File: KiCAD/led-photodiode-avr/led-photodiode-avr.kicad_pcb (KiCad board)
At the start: 4 copper layers, 68.6 x 80 mm, 68 parts, among them J1 Screw_Terminal_01x02, J2 Conn_02x08_Odd_Even, J3 ISP, J4 Conn_01x06_Pin, Q1 TTC1949, Q2 TTC1949, Q3 TTC1949, Q4 TTC1949, U1 REF3040AIDBZT, U10 AZ1117CH2-5.0, U2 AZ1117CH2-5.0, U3 OPA365xxD, U5 DDC112, U6 LTC1380, U7 ATmega328-A, U8 OPA365AIDR, U9 LTC2631, Y1 CO_16MHZ

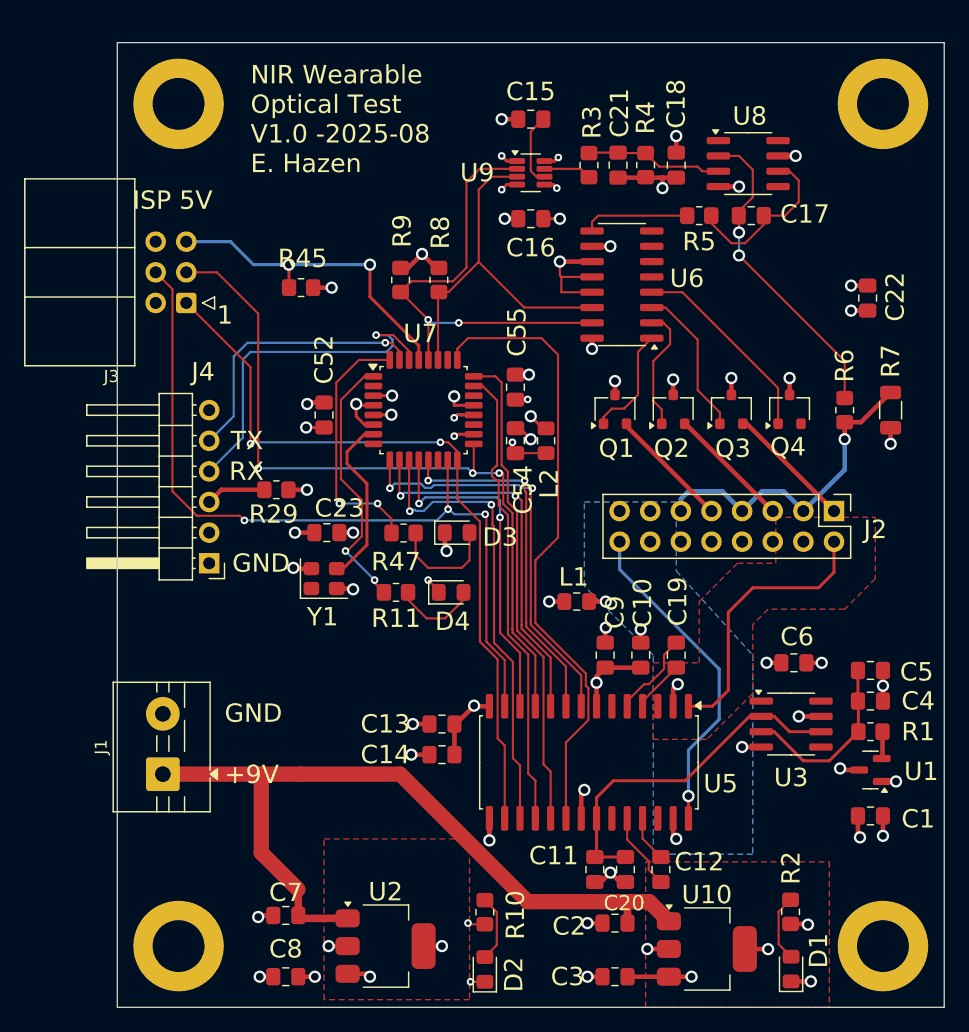
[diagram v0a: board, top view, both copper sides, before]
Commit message: more tests
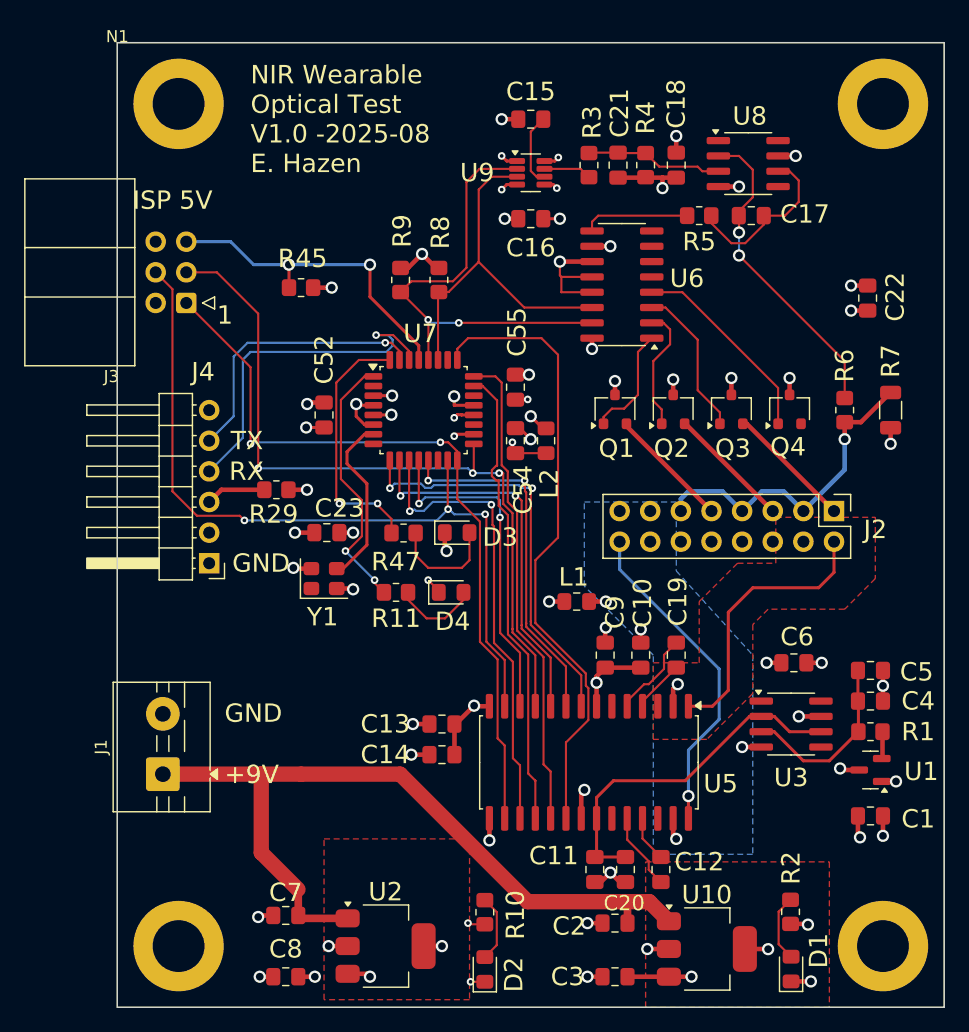
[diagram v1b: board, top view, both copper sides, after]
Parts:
- added N1: Optical_PCB, optical_pcb_model:optical_pcb, F.Cu at (116.8, 57.1)
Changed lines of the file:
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@@
 		)
 	)
+	(footprint "optical_pcb_model:optical_pcb"
+		(layer "F.Cu")
+		(at 116.84 57.15)
+		(property "Reference" "N1"
+			(at 0 -0.5 0)
+			(unlocked yes)
+			(layer "F.SilkS")
+			(effects
+				(font
+					(size 1 1)
+					(thickness 0.1)
+				)
+			)
+		)
+		(property "Value" "Optical_PCB"
+			(at 0 1 0)
+			(unlocked yes)
+			(layer "F.Fab")
+			(effects
+				(font
+					(size 1 1)
+					(thickness 0.15)
+				)
+			)
+		)
+		(property "Datasheet" "~"
+			(at 0 0 0)
+			(unlocked yes)
+			(layer "F.Fab")
+			(hide yes)
+			(effects
+				(font
+					(size 1 1)
+					(thickness 0.15)
+				)
+			)
+		)
+		(property "Description" "Housing"
+			(at 0 0 0)
+			(unlocked yes)
+			(layer "F.Fab")
+			(hide yes)
+			(effects
+				(font
+					(size 1 1)
+					(thickness 0.15)
+				)
+			)
+		)
+		(property ki_fp_filters "Enclosure* Housing*")
+		(sheetname "/")
+		(sheetfile "led-photodiode-avr.kicad_sch")
+		(attr smd)
+		(fp_rect
+			(start 0 0)
+			(end 68.58 80.01)
+			(stroke
+				(width 0.1)
+				(type default)
+			)
+			(fill no)
+			(layer "F.SilkS")
+		)
+		(fp_rect
+			(start 0 0)
+			(end 68.58 80.01)
+			(stroke
+				(width 0.1)
+				(type default)
+			)
+			(fill no)
+			(layer "User.2")
+		)
+		(fp_text user "${REFERENCE}"
+			(at 0 2.5 0)
+			(unlocked yes)
+			(layer "F.Fab")
+			(effects
+				(font
+					(size 1 1)
+					(thickness 0.15)
+				)
+			)
+		)
+		(pad "1" thru_hole circle
+			(at 5.08 5.08)
+			(size 4.572 4.572)
+			(drill 3.175)
+			(layers "*.Cu" "*.Mask")
+			(remove_unused_layers no)
+		)
+		(embedded_fonts no)
+		(model "${KIPRJMOD}/models/optical-carrier.wrl"
+			(offset
+				(xyz -169.545 55.88 12.065)
+			)
+			(scale
+				(xyz 0.392 0.392 0.392)
+			)
+			(rotate
+				(xyz -0 -0 -0)
+			)
+		)
+	)
 	(footprint "LED_SMD:LED_0805_2012Metric_Pad1.15x1.40mm_HandSolder"
 		(layer "F.Cu")
@@
 			(roundrect_rratio 0.25)
 			(net 6 "VCC")
-			(pinfunction "REF_SEL")
+			(pinfunction "CA1")
 			(pintype "passive")
 		)
@@
 		(layer "User.2")
 		(pts
+			(xy 116.84 57.15) (xy 121.92 62.23)
+		)
+		(height -6.604)
+		(orientation 0)
+		(format
+			(prefix "")
+			(suffix "")
+			(units 3)
+			(units_format 0)
+			(precision 4)
+			(suppress_zeroes yes)
+		)
+		(style
+			(thickness 0.1)
+			(arrow_length 1.27)
+			(text_position_mode 0)
+			(arrow_direction outward)
+			(extension_height 0.58642)
+			(extension_offset 0.5)
+			(keep_text_aligned yes)
+		)
+		(gr_text "0.2"
+			(at 119.38 49.396 0)
+			(layer "User.2")
+			(effects
+				(font
+					(size 1 1)
+					(thickness 0.15)
+				)
+			)
+		)
+	)
+	(dimension
+		(type orthogonal)
+		(layer "User.2")
+		(pts
 			(xy 180.34 62.23) (xy 180.34 132.08)
 		)
@@
 			(layer "User.2")
 			(effects
+				(font
+					(size 1 1)
+					(thickness 0.15)
+				)
+			)
+		)
+	)
+	(dimension
+		(type orthogonal)
+		(layer "User.2")
+		(pts
+			(xy 116.84 57.15) (xy 121.92 62.23)
+		)
+		(height -3.429)
+		(orientation 1)
+		(format
+			(prefix "")
+			(suffix "")
+			(units 3)
+			(units_format 0)
+			(precision 4)
+			(suppress_zeroes yes)
+		)
+		(style
+			(thickness 0.1)
+			(arrow_length 1.27)
+			(text_position_mode 0)
+			(arrow_direction outward)
+			(extension_height 0.58642)
+			(extension_offset 0.5)
+			(keep_text_aligned yes)
+		)
+		(gr_text "0.2"
+			(at 112.261 59.69 90)
+			(layer "User.2")
+			(effects
